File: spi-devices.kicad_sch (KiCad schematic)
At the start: 15 parts, among them U5 IIM-42652, U8 ICE5LP1K-SG48

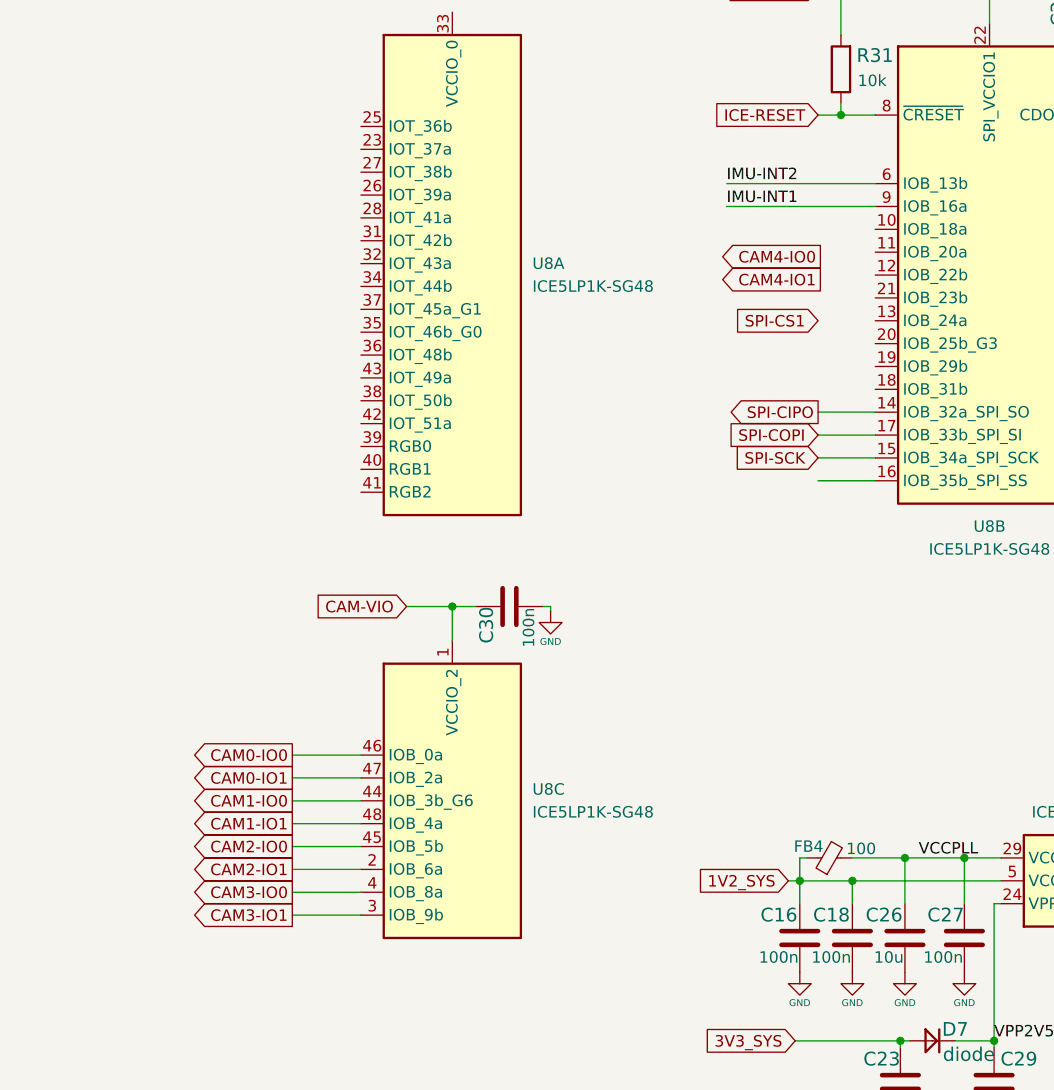
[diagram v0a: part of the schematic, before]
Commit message: Checkpoint
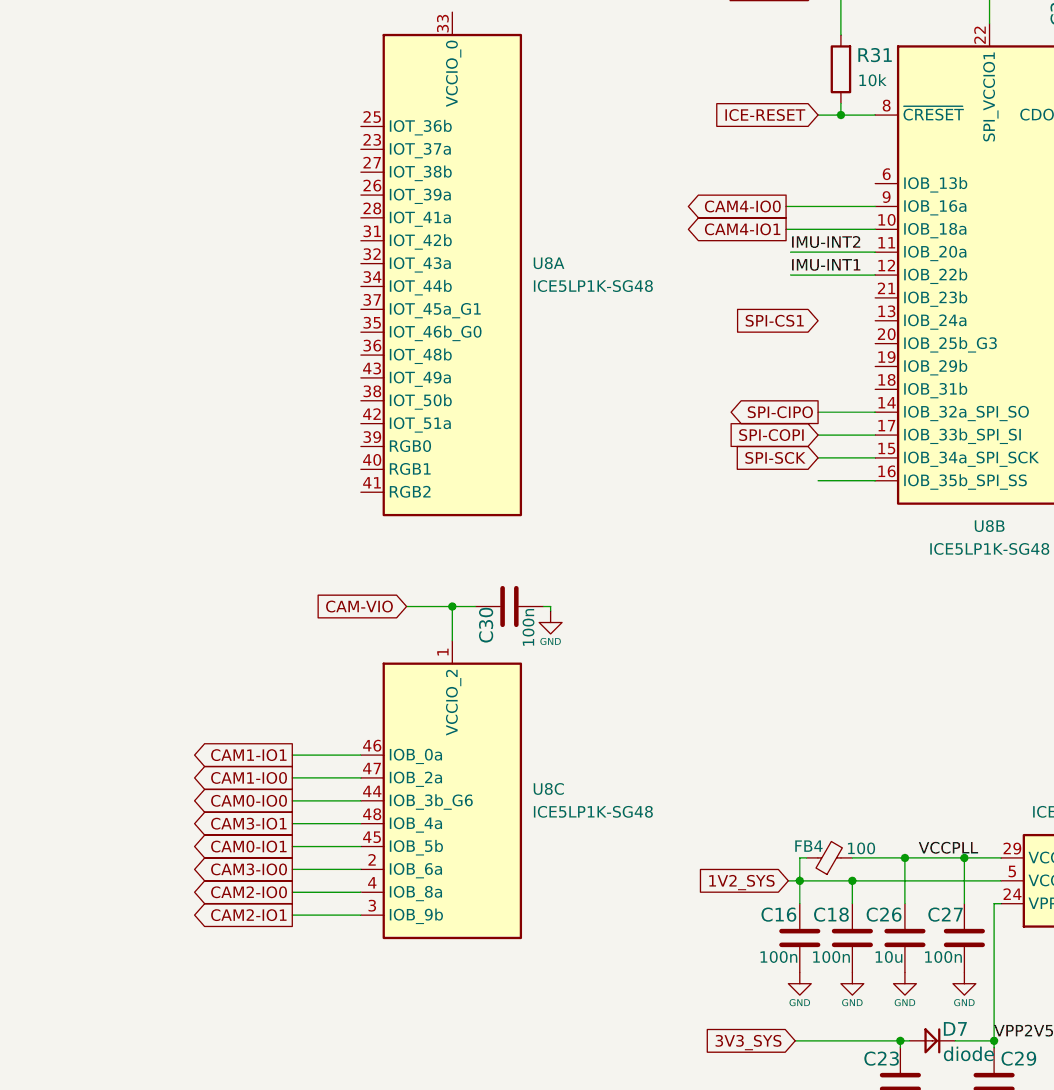
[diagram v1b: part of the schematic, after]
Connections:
- net CAM0-IO0: now also U8.44 (IOB_3b_G6); no longer U8.46 (IOB_0a)
- net CAM0-IO1: now also U8.45 (IOB_5b); no longer U8.47 (IOB_2a)
- net CAM1-IO0: now also U8.47 (IOB_2a); no longer U8.44 (IOB_3b_G6)
- net CAM1-IO1: now also U8.46 (IOB_0a); no longer U8.48 (IOB_4a)
- net CAM2-IO0: now also U8.4 (IOB_8a); no longer U8.45 (IOB_5b)
- net CAM2-IO1: now also U8.3 (IOB_9b); no longer U8.2 (IOB_6a)
- net CAM3-IO0: now also U8.2 (IOB_6a); no longer U8.4 (IOB_8a)
- net CAM3-IO1: now also U8.48 (IOB_4a); no longer U8.3 (IOB_9b)
- net CAM4-IO0: now also U8.9 (IOB_16a)
- net CAM4-IO1: now also U8.10 (IOB_18a)
- net IMU-INT1: now also U8.12 (IOB_22b); no longer U8.9 (IOB_16a)
- net IMU-INT2: now also U8.11 (IOB_20a); no longer U8.6 (IOB_13b)
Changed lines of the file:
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@@
+    (stroke (width 0) (type default) (color 0 0 0 0))
+  )
+  (wire (pts (xy 222.504 64.77) (xy 232.41 64.77))
     (stroke (width 0) (type default) (color 0 0 0 0))
   )
@@
     (stroke (width 0) (type default) (color 0 0 0 0))
   )
+  (wire (pts (xy 222.504 62.23) (xy 232.41 62.23))
+    (stroke (width 0) (type default) (color 0 0 0 0))
+  )
   (wire (pts (xy 97.155 52.705) (xy 97.155 54.61))
     (stroke (width 0) (type default) (color 0 0 0 0))
@@
     (stroke (width 0) (type default) (color 0 0 0 0))
   )
-  (wire (pts (xy 215.9 59.69) (xy 232.41 59.69))
+  (wire (pts (xy 223.012 67.31) (xy 232.41 67.31))
     (stroke (width 0) (type default) (color 0 0 0 0))
   )
@@
     (stroke (width 0) (type default) (color 0 0 0 0))
   )
-  (wire (pts (xy 215.9 62.23) (xy 232.41 62.23))
+  (wire (pts (xy 223.012 69.85) (xy 232.41 69.85))
     (stroke (width 0) (type default) (color 0 0 0 0))
   )
@@
     (stroke (width 0) (type default) (color 0 0 0 0))
   )
-  (label "IMU-INT2" (at 215.9 59.69 0)
-    (effects (font (size 1.27 1.27)) (justify left bottom))
-  )
-  (label "IMU-INT1" (at 215.9 62.23 0)
+  (label "IMU-INT2" (at 223.012 67.31 0)
+    (effects (font (size 1.27 1.27)) (justify left bottom))
+  )
+  (label "IMU-INT1" (at 223.012 69.85 0)
     (effects (font (size 1.27 1.27)) (justify left bottom))
   )
@@
     )
   )
-  (global_label "CAM2-IO0" (shape output) (at 167.64 133.35 180) (fields_autoplaced)
-    (effects (font (size 1.27 1.27)) (justify right))
-    (property "Intersheet References" "${INTERSHEET_REFS}" (id 0) (at 155.5791 133.2706 0)
-      (effects (font (size 1.27 1.27)) (justify right) hide)
-    )
-  )
-  (global_label "CAM3-IO1" (shape output) (at 167.64 140.97 180) (fields_autoplaced)
-    (effects (font (size 1.27 1.27)) (justify right))
-    (property "Intersheet References" "${INTERSHEET_REFS}" (id 0) (at 155.5791 140.8906 0)
-      (effects (font (size 1.27 1.27)) (justify right) hide)
-    )
-  )
-  (global_label "CAM3-IO0" (shape output) (at 167.64 138.43 180) (fields_autoplaced)
+  (global_label "CAM2-IO0" (shape output) (at 167.64 138.43 180) (fields_autoplaced)
     (effects (font (size 1.27 1.27)) (justify right))
     (property "Intersheet References" "${INTERSHEET_REFS}" (id 0) (at 155.5791 138.3506 0)
+      (effects (font (size 1.27 1.27)) (justify right) hide)
+    )
+  )
+  (global_label "CAM3-IO1" (shape output) (at 167.64 130.81 180) (fields_autoplaced)
+    (effects (font (size 1.27 1.27)) (justify right))
+    (property "Intersheet References" "${INTERSHEET_REFS}" (id 0) (at 155.5791 130.7306 0)
+      (effects (font (size 1.27 1.27)) (justify right) hide)
+    )
+  )
+  (global_label "CAM3-IO0" (shape output) (at 167.64 135.89 180) (fields_autoplaced)
+    (effects (font (size 1.27 1.27)) (justify right))
+    (property "Intersheet References" "${INTERSHEET_REFS}" (id 0) (at 155.5791 135.8106 0)
       (effects (font (size 1.27 1.27)) (justify right) hide)
     )
@@
     )
   )
-  (global_label "CAM4-IO0" (shape output) (at 226.314 67.818 180) (fields_autoplaced)
-    (effects (font (size 1.27 1.27)) (justify right))
-    (property "Intersheet References" "${INTERSHEET_REFS}" (id 0) (at 214.2531 67.7386 0)
-      (effects (font (size 1.27 1.27)) (justify right) hide)
-    )
-  )
-  (global_label "CAM2-IO1" (shape output) (at 167.64 135.89 180) (fields_autoplaced)
-    (effects (font (size 1.27 1.27)) (justify right))
-    (property "Intersheet References" "${INTERSHEET_REFS}" (id 0) (at 155.5791 135.8106 0)
+  (global_label "CAM4-IO0" (shape output) (at 222.504 62.23 180) (fields_autoplaced)
+    (effects (font (size 1.27 1.27)) (justify right))
+    (property "Intersheet References" "${INTERSHEET_REFS}" (id 0) (at 210.4431 62.1506 0)
+      (effects (font (size 1.27 1.27)) (justify right) hide)
+    )
+  )
+  (global_label "CAM2-IO1" (shape output) (at 167.64 140.97 180) (fields_autoplaced)
+    (effects (font (size 1.27 1.27)) (justify right))
+    (property "Intersheet References" "${INTERSHEET_REFS}" (id 0) (at 155.5791 140.8906 0)
       (effects (font (size 1.27 1.27)) (justify right) hide)
     )
@@
     )
   )
-  (global_label "CAM0-IO0" (shape output) (at 167.64 123.19 180) (fields_autoplaced)
+  (global_label "CAM0-IO0" (shape output) (at 167.64 128.27 180) (fields_autoplaced)
+    (effects (font (size 1.27 1.27)) (justify right))
+    (property "Intersheet References" "${INTERSHEET_REFS}" (id 0) (at 155.5791 128.1906 0)
+      (effects (font (size 1.27 1.27)) (justify right) hide)
+    )
+  )
+  (global_label "CAM-VIO" (shape input) (at 180.34 106.68 180) (fields_autoplaced)
+    (effects (font (size 1.27 1.27)) (justify right))
+    (property "Intersheet References" "${INTERSHEET_REFS}" (id 0) (at 169.6096 106.7594 0)
+      (effects (font (size 1.27 1.27)) (justify right) hide)
+    )
+  )
+  (global_label "ICE-RESET" (shape input) (at 226.06 52.07 180) (fields_autoplaced)
+    (effects (font (size 1.27 1.27)) (justify right))
+    (property "Intersheet References" "${INTERSHEET_REFS}" (id 0) (at 213.3944 51.9906 0)
+      (effects (font (size 1.27 1.27)) (justify right) hide)
+    )
+  )
+  (global_label "3V3_SYS" (shape input) (at 226.06 38.1 180) (fields_autoplaced)
+    (effects (font (size 1.27 1.27)) (justify right))
+    (property "Intersheet References" "${INTERSHEET_REFS}" (id 0) (at 215.7529 38.0206 0)
+      (effects (font (size 1.27 1.27)) (justify right) hide)
+    )
+  )
+  (global_label "SPI-COPI" (shape input) (at 226.06 87.63 180) (fields_autoplaced)
+    (effects (font (size 1.27 1.27)) (justify right))
+    (property "Intersheet References" "${INTERSHEET_REFS}" (id 0) (at 214.6039 87.5506 0)
+      (effects (font (size 1.27 1.27)) (justify right) hide)
+    )
+  )
+  (global_label "CAM1-IO0" (shape output) (at 167.64 125.73 180) (fields_autoplaced)
+    (effects (font (size 1.27 1.27)) (justify right))
+    (property "Intersheet References" "${INTERSHEET_REFS}" (id 0) (at 155.5791 125.6506 0)
+      (effects (font (size 1.27 1.27)) (justify right) hide)
+    )
+  )
+  (global_label "SPI-CS1" (shape input) (at 226.06 74.93 180) (fields_autoplaced)
+    (effects (font (size 1.27 1.27)) (justify right))
+    (property "Intersheet References" "${INTERSHEET_REFS}" (id 0) (at 215.3901 74.8506 0)
+      (effects (font (size 1.27 1.27)) (justify right) hide)
+    )
+  )
+  (global_label "CAM4-IO1" (shape output) (at 222.504 64.77 180) (fields_autoplaced)
+    (effects (font (size 1.27 1.27)) (justify right))
+    (property "Intersheet References" "${INTERSHEET_REFS}" (id 0) (at 210.4431 64.6906 0)
+      (effects (font (size 1.27 1.27)) (justify right) hide)
+    )
+  )
+  (global_label "CAM1-IO1" (shape output) (at 167.64 123.19 180) (fields_autoplaced)
     (effects (font (size 1.27 1.27)) (justify right))
     (property "Intersheet References" "${INTERSHEET_REFS}" (id 0) (at 155.5791 123.1106 0)
@@
     )
   )
-  (global_label "CAM-VIO" (shape input) (at 180.34 106.68 180) (fields_autoplaced)
-    (effects (font (size 1.27 1.27)) (justify right))
-    (property "Intersheet References" "${INTERSHEET_REFS}" (id 0) (at 169.6096 106.7594 0)
-      (effects (font (size 1.27 1.27)) (justify right) hide)
-    )
-  )
-  (global_label "ICE-RESET" (shape input) (at 226.06 52.07 180) (fields_autoplaced)
-    (effects (font (size 1.27 1.27)) (justify right))
-    (property "Intersheet References" "${INTERSHEET_REFS}" (id 0) (at 213.3944 51.9906 0)
-      (effects (font (size 1.27 1.27)) (justify right) hide)
-    )
-  )
-  (global_label "3V3_SYS" (shape input) (at 226.06 38.1 180) (fields_autoplaced)
-    (effects (font (size 1.27 1.27)) (justify right))
-    (property "Intersheet References" "${INTERSHEET_REFS}" (id 0) (at 215.7529 38.0206 0)
-      (effects (font (size 1.27 1.27)) (justify right) hide)
-    )
-  )
-  (global_label "SPI-COPI" (shape input) (at 226.06 87.63 180) (fields_autoplaced)
-    (effects (font (size 1.27 1.27)) (justify right))
-    (property "Intersheet References" "${INTERSHEET_REFS}" (id 0) (at 214.6039 87.5506 0)
-      (effects (font (size 1.27 1.27)) (justify right) hide)
-    )
-  )
-  (global_label "CAM1-IO0" (shape output) (at 167.64 128.27 180) (fields_autoplaced)
-    (effects (font (size 1.27 1.27)) (justify right))
-    (property "Intersheet References" "${INTERSHEET_REFS}" (id 0) (at 155.5791 128.1906 0)
-      (effects (font (size 1.27 1.27)) (justify right) hide)
-    )
-  )
-  (global_label "SPI-CS1" (shape input) (at 226.06 74.93 180) (fields_autoplaced)
-    (effects (font (size 1.27 1.27)) (justify right))
-    (property "Intersheet References" "${INTERSHEET_REFS}" (id 0) (at 215.3901 74.8506 0)
-      (effects (font (size 1.27 1.27)) (justify right) hide)
-    )
-  )
-  (global_label "CAM4-IO1" (shape output) (at 226.314 70.358 180) (fields_autoplaced)
-    (effects (font (size 1.27 1.27)) (justify right))
-    (property "Intersheet References" "${INTERSHEET_REFS}" (id 0) (at 214.2531 70.2786 0)
-      (effects (font (size 1.27 1.27)) (justify right) hide)
-    )
-  )
-  (global_label "CAM1-IO1" (shape output) (at 167.64 130.81 180) (fields_autoplaced)
-    (effects (font (size 1.27 1.27)) (justify right))
-    (property "Intersheet References" "${INTERSHEET_REFS}" (id 0) (at 155.5791 130.7306 0)
-      (effects (font (size 1.27 1.27)) (justify right) hide)
-    )
-  )
-  (global_label "CAM0-IO1" (shape output) (at 167.64 125.73 180) (fields_autoplaced)
-    (effects (font (size 1.27 1.27)) (justify right))
-    (property "Intersheet References" "${INTERSHEET_REFS}" (id 0) (at 155.5791 125.6506 0)
-      (effects (font (size 1.27 1.27)) (justify right) hide)
-    )
+  (global_label "CAM0-IO1" (shape output) (at 167.64 133.35 180) (fields_autoplaced)
+    (effects (font (size 1.27 1.27)) (justify right))
+    (property "Intersheet References" "${INTERSHEET_REFS}" (id 0) (at 155.5791 133.2706 0)
+      (effects (font (size 1.27 1.27)) (justify right) hide)
+    )
